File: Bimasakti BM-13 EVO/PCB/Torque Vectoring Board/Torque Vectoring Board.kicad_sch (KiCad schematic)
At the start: 30 parts, among them J1 SIGNAL 1, J2 SIGNAL 1, U3 SN65HVD230, U4 SN65HVD230, U5 ADS1115IDGS

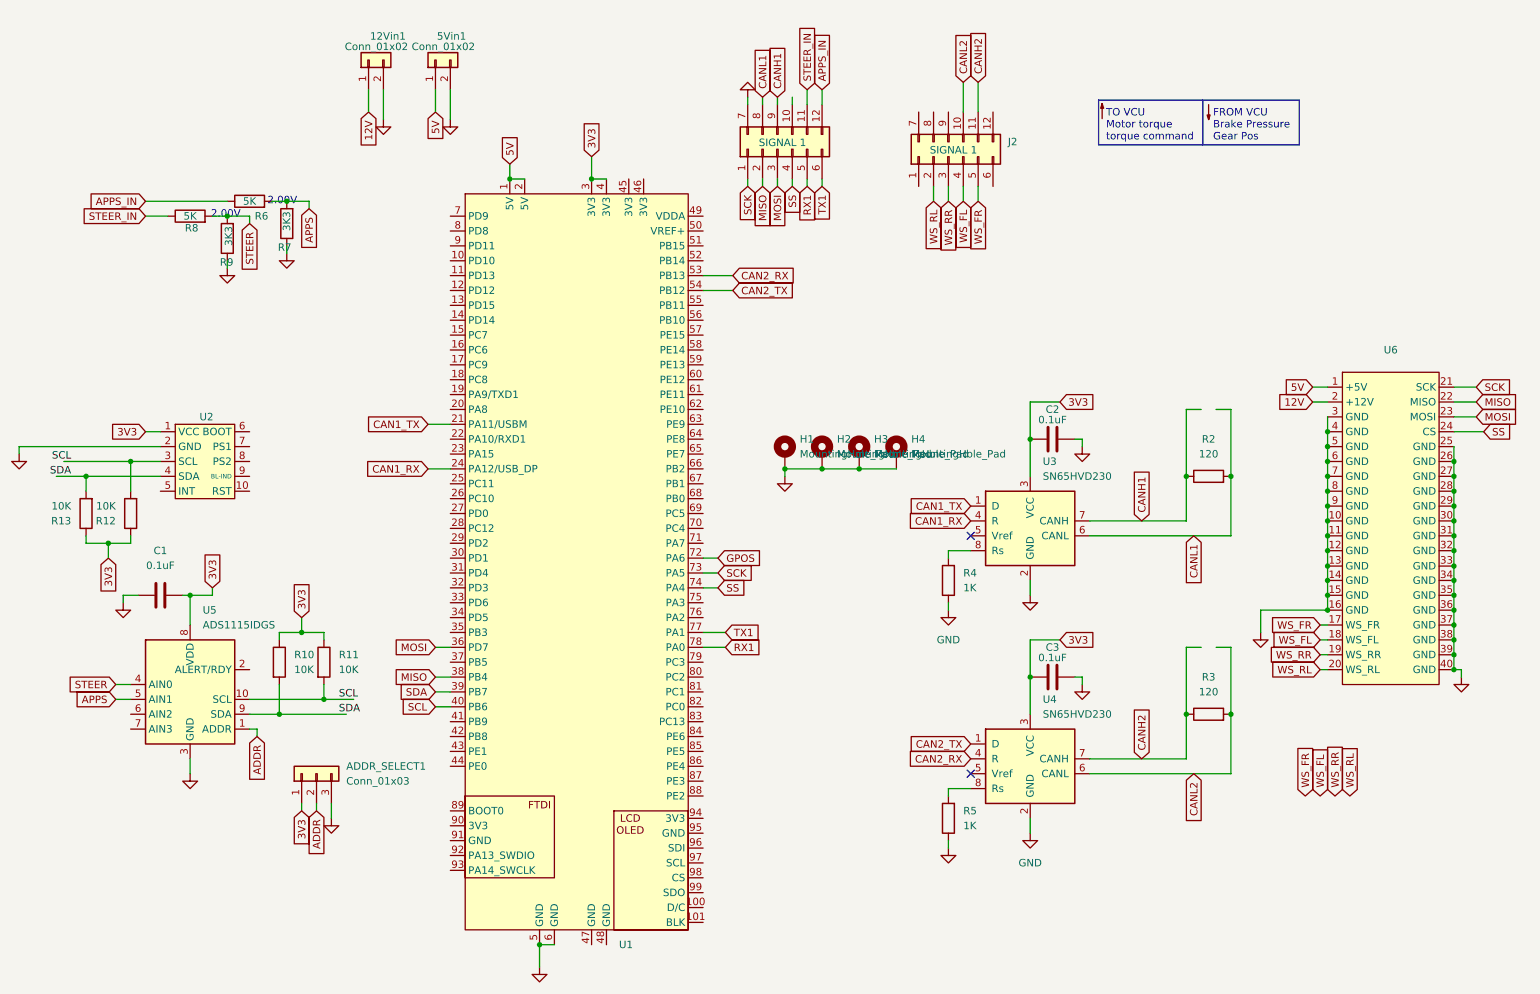
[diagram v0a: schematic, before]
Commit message: assembly kurang pneumatic, kurang wiring dudukan motherboard
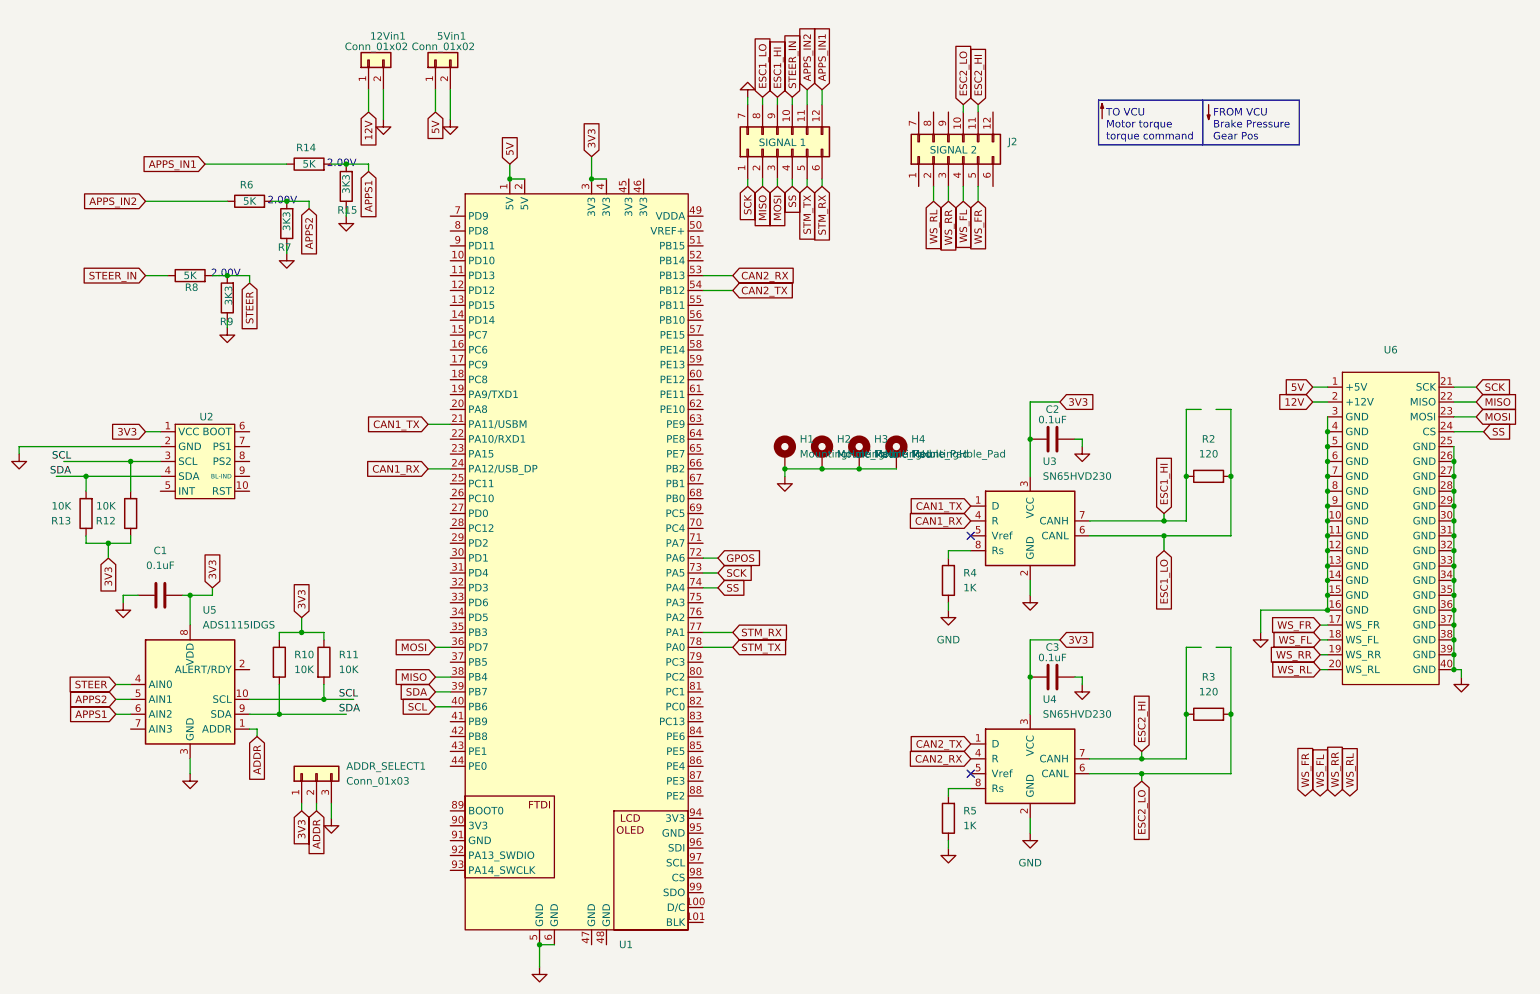
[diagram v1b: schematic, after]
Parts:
- added R14: 5K, Resistor_SMD:R_0805_2012Metric, symbol Device:R
- added R15: 3K3, Resistor_SMD:R_0805_2012Metric, symbol Device:R
- J2: value SIGNAL 1 -> SIGNAL 2
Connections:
- net GND: now also R15.1
- net STEER_IN: now also J1.10 (Pin_10); no longer J1.11 (Pin_11)
- net APPS1: now reaches U5.6 (AIN2)
- net APPS1: now also R14.2, R15.2
- net APPS renamed APPS2
- net APPS_IN renamed APPS_IN1
- net APPS_IN1: now also R14.1; no longer R6.1
- net CANH1 renamed ESC1_HI
- net CANH2 renamed ESC2_HI
- net CANL1 renamed ESC1_LO
- net CANL2 renamed ESC2_LO
- net RX1 renamed STM_TX
- net TX1 renamed STM_RX
- new net APPS_IN2: J1.11 (Pin_11), R6.1
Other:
- moved on the sheet: R8, R9
